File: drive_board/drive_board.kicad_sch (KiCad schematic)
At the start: 13 parts, among them J1 RJ45_LED_Shielded, J3 Conn_01x02_Pin, J4 Conn_01x02_Pin, J5 Conn_01x02_Pin, J6 Conn_01x02_Pin, J7 Conn_01x02_Pin, U3 SN65HVD232

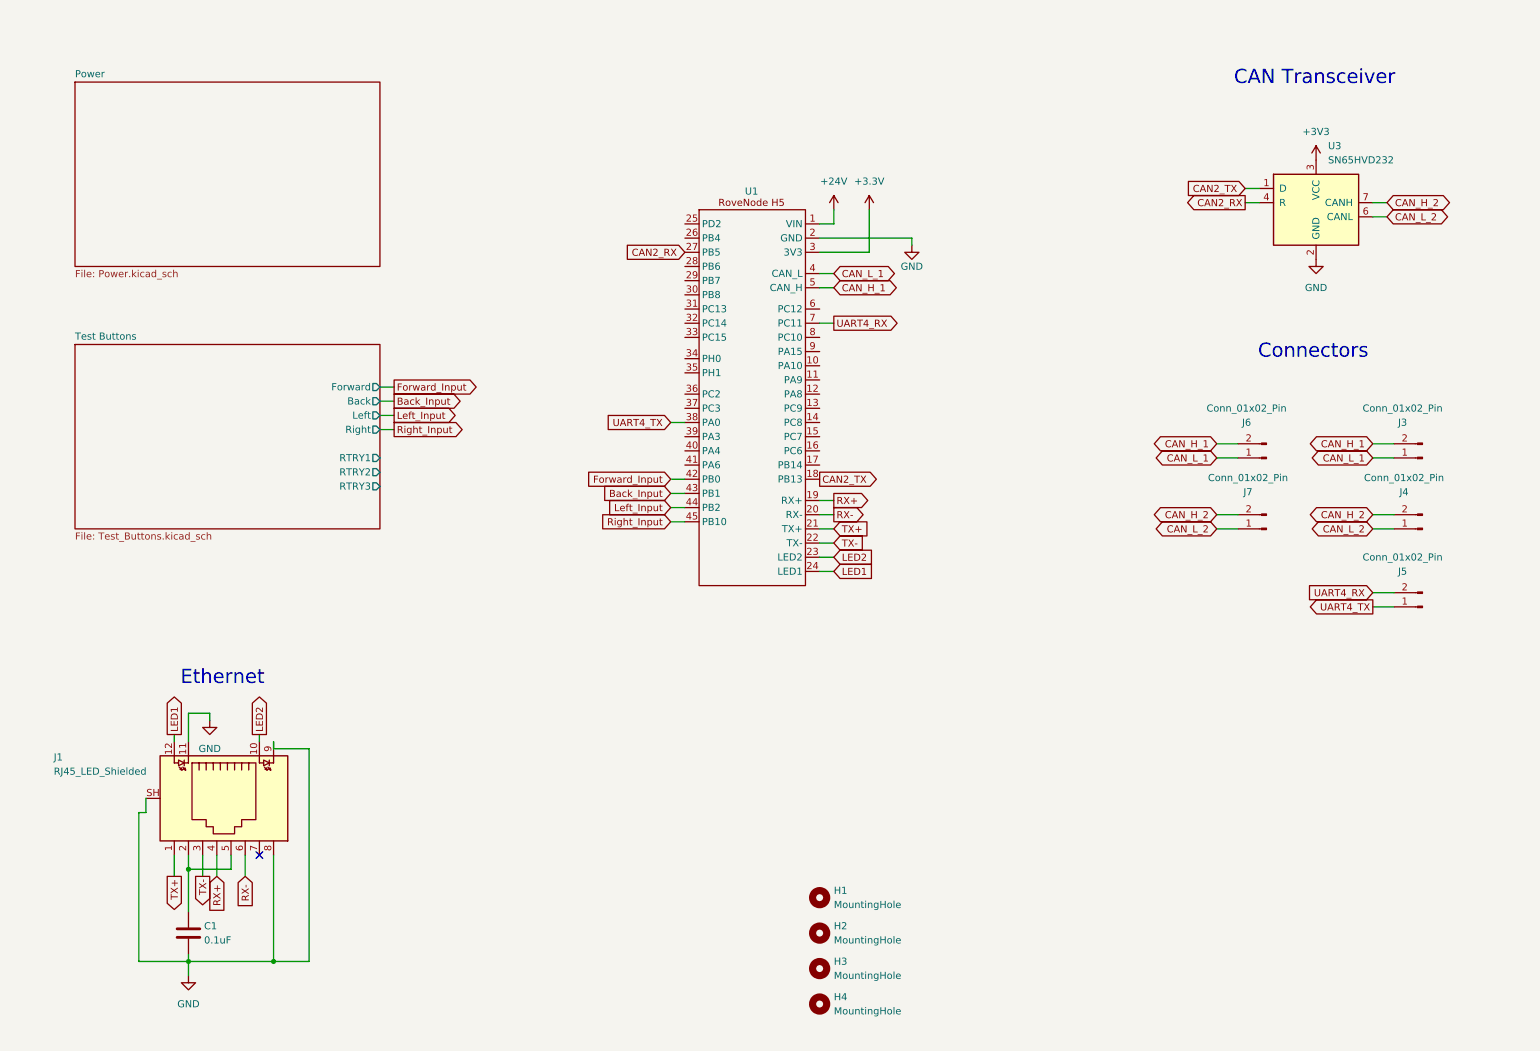
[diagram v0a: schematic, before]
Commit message: Finish schematic
- Finished requirements
- Cleaned up and organized some stuff
- Can still clean up a little more
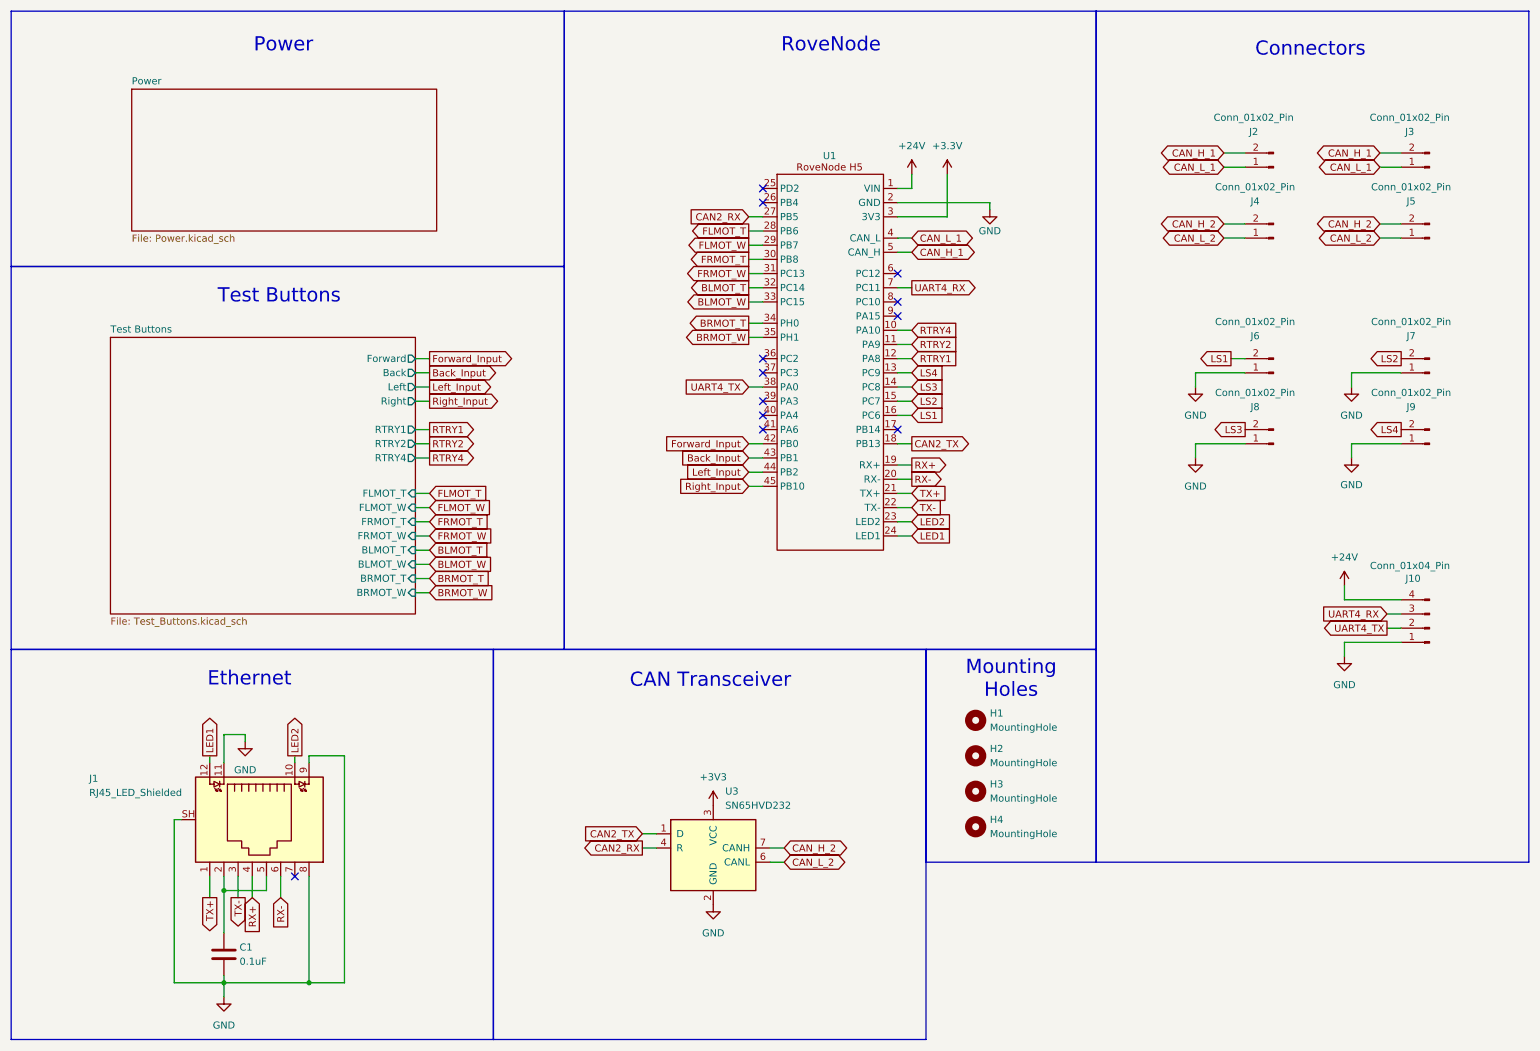
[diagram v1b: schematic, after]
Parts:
- removed J5: Conn_01x02_Pin, Package_DFN_QFN:QFN-20-1EP_5x5mm_P0.65mm_EP3.35x3.35mm, symbol Connector:Conn_01x02_Pin
- added J10: Conn_01x04_Pin, Package_DIP:DIP-20_W7.62mm, symbol Connector:Conn_01x04_Pin
- added J6, J7, J8, J9: Conn_01x02_Pin, Package_DFN_QFN:QFN-20-1EP_5x5mm_P0.65mm_EP3.35x3.35mm, symbol Connector:Conn_01x02_Pin
- renumbered J6 to J2, J7 to J4, J4 to J5
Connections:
- net +24V: now also J10.4 (Pin_4)
- net GND: now also J10.1 (Pin_1), J6.1 (Pin_1), J7.1 (Pin_1), J8.1 (Pin_1), J9.1 (Pin_1)
- net UART4_RX: now also J10.3 (Pin_3)
- net UART4_TX: now also J10.2 (Pin_2)
- net RTRY4: now reaches U1.10 (PA10)
- net RTRY2: now reaches U1.11 (PA9)
- net RTRY1: now reaches U1.12 (PA8)
- net LS4: now reaches U1.13 (PC9)
- net LS4: now also J9.2 (Pin_2)
- net LS3: now reaches U1.14 (PC8)
- net LS3: now also J8.2 (Pin_2)
- net LS2: now reaches U1.15 (PC7)
- net LS2: now also J7.2 (Pin_2)
- net LS1: now reaches U1.16 (PC6)
- net LS1: now also J6.2 (Pin_2)
- net FLMOT_T: now reaches U1.28 (PB6)
- net FLMOT_W: now reaches U1.29 (PB7)
- net FRMOT_T: now reaches U1.30 (PB8)
- net FRMOT_W: now reaches U1.31 (PC13)
- net BLMOT_T: now reaches U1.32 (PC14)
- net BLMOT_W: now reaches U1.33 (PC15)
- net BRMOT_T: now reaches U1.34 (PH0)
- net BRMOT_W: now reaches U1.35 (PH1)
- no-connect marks 1 -> 12
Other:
- sheet Test Buttons ports: added BLMOT_T, BLMOT_W, BRMOT_T, BRMOT_W, FLMOT_T, FLMOT_W, FRMOT_T, FRMOT_W, RTRY4; removed RTRY3
- note added: "Mounting Holes"
- note added: "Power"
- note added: "RoveNode"
- note added: "Test Buttons"
- moved on the sheet: C1, H1, H2, H3, H4, J1, J2, J3, J4, J5, U1, U3
